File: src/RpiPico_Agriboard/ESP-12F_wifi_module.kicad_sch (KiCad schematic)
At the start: 12 parts, among them J27 Conn_02x05_Odd_Even, SW3 SW_Push, SW4 SW_Push, U4 ESP-12F

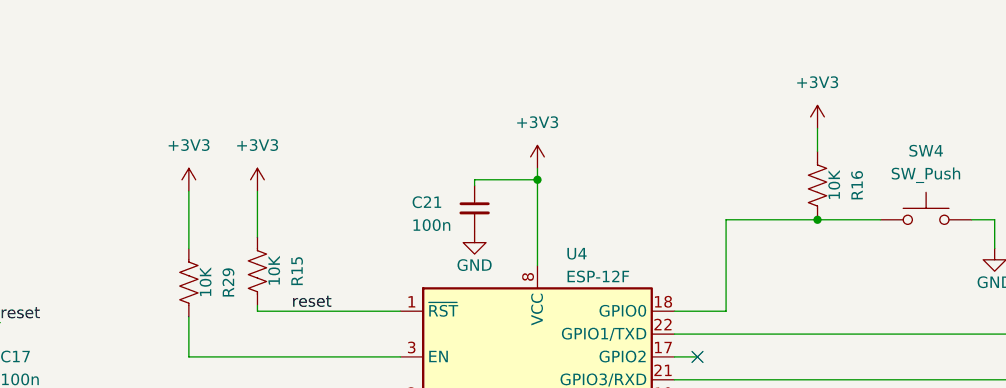
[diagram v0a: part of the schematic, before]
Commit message: schematic updates completed
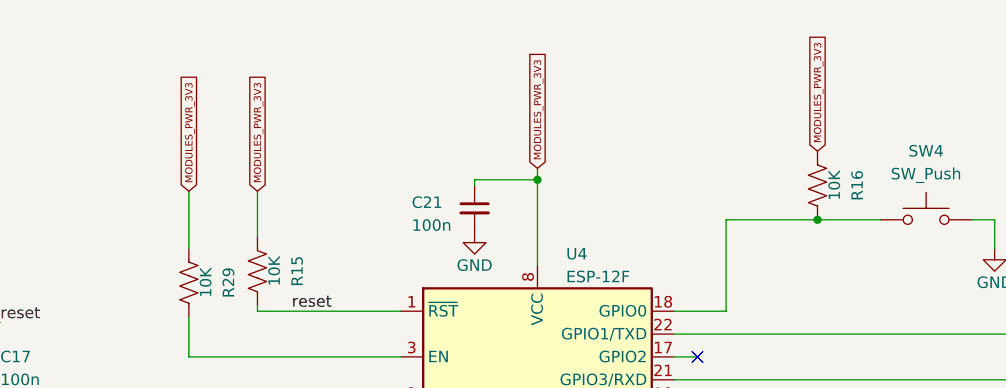
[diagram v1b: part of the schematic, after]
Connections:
- net +3V3: no longer C21.1, R15.1, R16.1, R29.1, U4.8 (VCC)
- new net MODULES_PWR_3V3: C21.1, R15.1, R16.1, R29.1, U4.8 (VCC)
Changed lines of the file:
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@@
-    (stroke (width 0) (type default))
-  )
-  (wire (pts (xy 170.815 45.72) (xy 170.815 48.26))
     (stroke (width 0) (type default))
   )
@@
     (effects (font (size 1.27 1.27)) (justify left bottom))
   )
+  (global_label "MODULES_PWR_3V3" (shape input) (at 100.965 52.705 90) (fields_autoplaced)
+    (effects (font (size 0.8 0.8)) (justify left))
+    (property "Intersheetrefs" "${INTERSHEET_REFS}" (at 100.965 39.4081 90)
+      (effects (font (size 1.27 1.27)) (justify left) hide)
+    )
+  )
+  (global_label "MODULES_PWR_3V3" (shape input) (at 170.815 48.26 90) (fields_autoplaced)
+    (effects (font (size 0.8 0.8)) (justify left))
+    (property "Intersheetrefs" "${INTERSHEET_REFS}" (at 170.815 34.9631 90)
+      (effects (font (size 1.27 1.27)) (justify left) hide)
+    )
+  )
+  (global_label "MODULES_PWR_3V3" (shape input) (at 139.7 50.165 90) (fields_autoplaced)
+    (effects (font (size 0.8 0.8)) (justify left))
+    (property "Intersheetrefs" "${INTERSHEET_REFS}" (at 139.7 36.8681 90)
+      (effects (font (size 1.27 1.27)) (justify left) hide)
+    )
+  )
+  (global_label "MODULES_PWR_3V3" (shape input) (at 108.585 52.705 90) (fields_autoplaced)
+    (effects (font (size 0.8 0.8)) (justify left))
+    (property "Intersheetrefs" "${INTERSHEET_REFS}" (at 108.585 39.4081 90)
+      (effects (font (size 1.27 1.27)) (justify left) hide)
+    )
+  )
   (hierarchical_label "ESP8266_RX_out" (shape input) (at 217.17 106.045 0) (fields_autoplaced)
     (effects (font (size 1.27 1.27) bold) (justify left))
@@
   (hierarchical_label "ESP8266_TX_out" (shape input) (at 217.17 100.965 0) (fields_autoplaced)
     (effects (font (size 1.27 1.27) bold) (justify left))
-  )
-  (symbol (lib_id "power:+3V3") (at 108.585 52.705 0) (unit 1)
-    (in_bom yes) (on_board yes) (dnp no) (fields_autoplaced)
-    (property "Reference" "#PWR040" (at 108.585 56.515 0)
-      (effects (font (size 1.27 1.27)) hide)
-    )
-    (property "Value" "+3V3" (at 108.585 47.625 0)
-      (effects (font (size 1.27 1.27)))
-    )
-    (property "Footprint" "" (at 108.585 52.705 0)
-      (effects (font (size 1.27 1.27)) hide)
-    )
-    (property "Datasheet" "" (at 108.585 52.705 0)
-      (effects (font (size 1.27 1.27)) hide)
-    )
-    (pin "1")
-    (instances
-      (project "RpiPico_Agriboard"
-        (path "/c2474b65-c0e8-4987-86b2-fddddd4113dc/24a6f6dd-59ed-4a3f-ab3f-0a381255370f/72a22278-332d-4fac-9f87-e146604ac9df"
-          (reference "#PWR040") (unit 1)
-        )
-      )
-    )
-  )
-  (symbol (lib_id "power:+3V3") (at 100.965 52.705 0) (unit 1)
-    (in_bom yes) (on_board yes) (dnp no) (fields_autoplaced)
-    (property "Reference" "#PWR039" (at 100.965 56.515 0)
-      (effects (font (size 1.27 1.27)) hide)
-    )
-    (property "Value" "+3V3" (at 100.965 47.625 0)
-      (effects (font (size 1.27 1.27)))
-    )
-    (property "Footprint" "" (at 100.965 52.705 0)
-      (effects (font (size 1.27 1.27)) hide)
-    )
-    (property "Datasheet" "" (at 100.965 52.705 0)
-      (effects (font (size 1.27 1.27)) hide)
-    )
-    (pin "1")
-    (instances
-      (project "RpiPico_Agriboard"
-        (path "/c2474b65-c0e8-4987-86b2-fddddd4113dc/24a6f6dd-59ed-4a3f-ab3f-0a381255370f/72a22278-332d-4fac-9f87-e146604ac9df"
-          (reference "#PWR039") (unit 1)
-        )
-      )
-    )
   )
   (symbol (lib_id "Device:R_US") (at 108.585 61.595 0) (unit 1)
@@
         (path "/c2474b65-c0e8-4987-86b2-fddddd4113dc/24a6f6dd-59ed-4a3f-ab3f-0a381255370f/72a22278-332d-4fac-9f87-e146604ac9df"
           (reference "TP_rx1") (unit 1)
-        )
-      )
-    )
-  )
-  (symbol (lib_id "power:+3V3") (at 139.7 50.165 0) (unit 1)
-    (in_bom yes) (on_board yes) (dnp no) (fields_autoplaced)
-    (property "Reference" "#PWR041" (at 139.7 53.975 0)
-      (effects (font (size 1.27 1.27)) hide)
-    )
-    (property "Value" "+3V3" (at 139.7 45.085 0)
-      (effects (font (size 1.27 1.27)))
-    )
-    (property "Footprint" "" (at 139.7 50.165 0)
-      (effects (font (size 1.27 1.27)) hide)
-    )
-    (property "Datasheet" "" (at 139.7 50.165 0)
-      (effects (font (size 1.27 1.27)) hide)
-    )
-    (pin "1")
-    (instances
-      (project "RpiPico_Agriboard"
-        (path "/c2474b65-c0e8-4987-86b2-fddddd4113dc/24a6f6dd-59ed-4a3f-ab3f-0a381255370f/72a22278-332d-4fac-9f87-e146604ac9df"
-          (reference "#PWR041") (unit 1)
         )
       )
@@
         )
       )
-    )
-  )
-  (symbol (lib_id "power:+3V3") (at 170.815 45.72 0) (unit 1)
-    (in_bom yes) (on_board yes) (dnp no) (fields_autoplaced)
-    (property "Reference" "#PWR043" (at 170.815 49.53 0)
-      (effects (font (size 1.27 1.27)) hide)
-    )
-    (property "Value" "+3V3" (at 170.815 40.64 0)
-      (effects (font (size 1.27 1.27)))
-    )
-    (property "Footprint" "" (at 170.815 45.72 0)
-      (effects (font (size 1.27 1.27)) hide)
-    )
-    (property "Datasheet" "" (at 170.815 45.72 0)
-      (effects (font (size 1.27 1.27)) hide)
-    )
-    (pin "1")
-    (instances
-      (project "RpiPico_Agriboard"
-        (path "/c2474b65-c0e8-4987-86b2-fddddd4113dc/24a6f6dd-59ed-4a3f-ab3f-0a381255370f/72a22278-332d-4fac-9f87-e146604ac9df"
-          (reference "#PWR043") (unit 1)
-        )
-      )
